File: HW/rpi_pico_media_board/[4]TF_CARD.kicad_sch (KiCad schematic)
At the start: 16 parts, among them J6 TF-01A

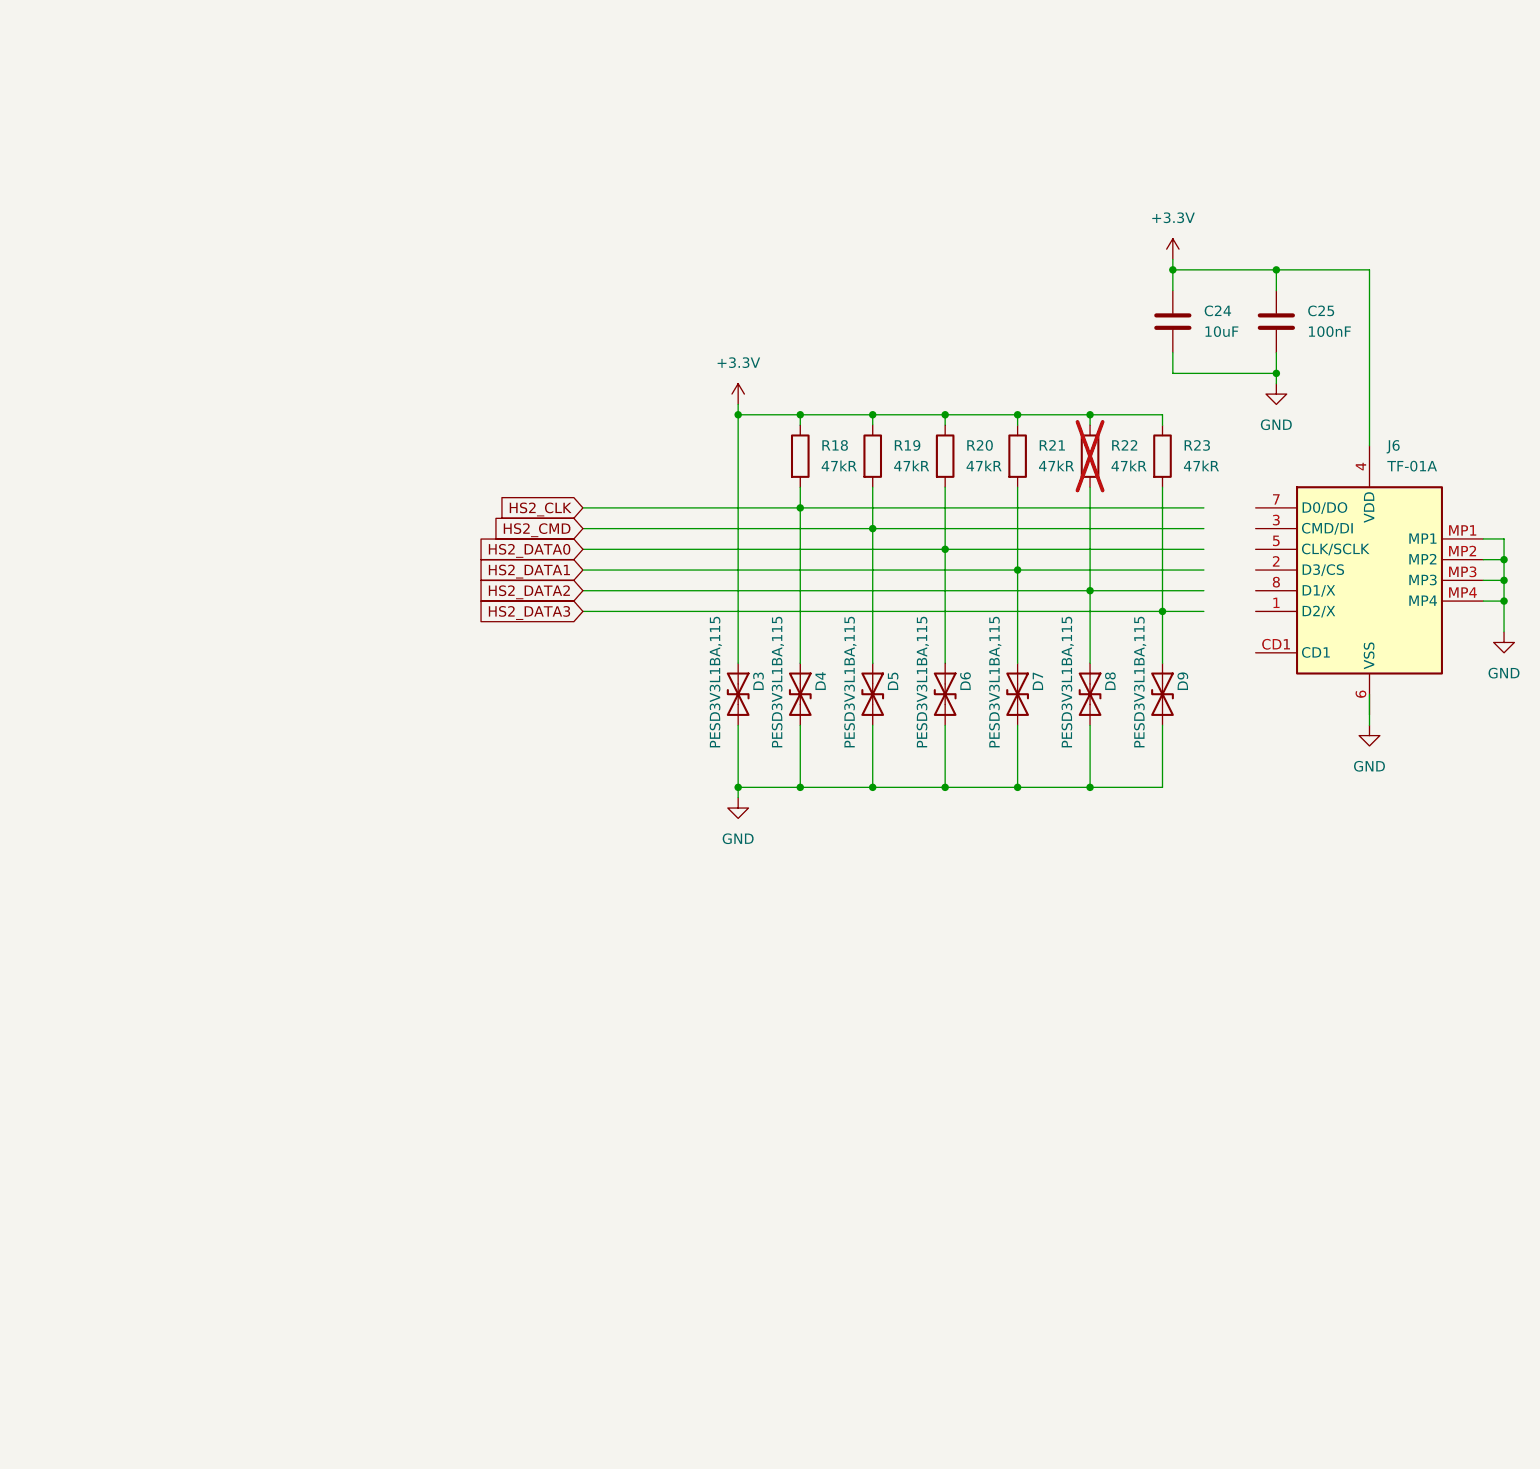
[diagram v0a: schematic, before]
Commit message: Scheme improvements
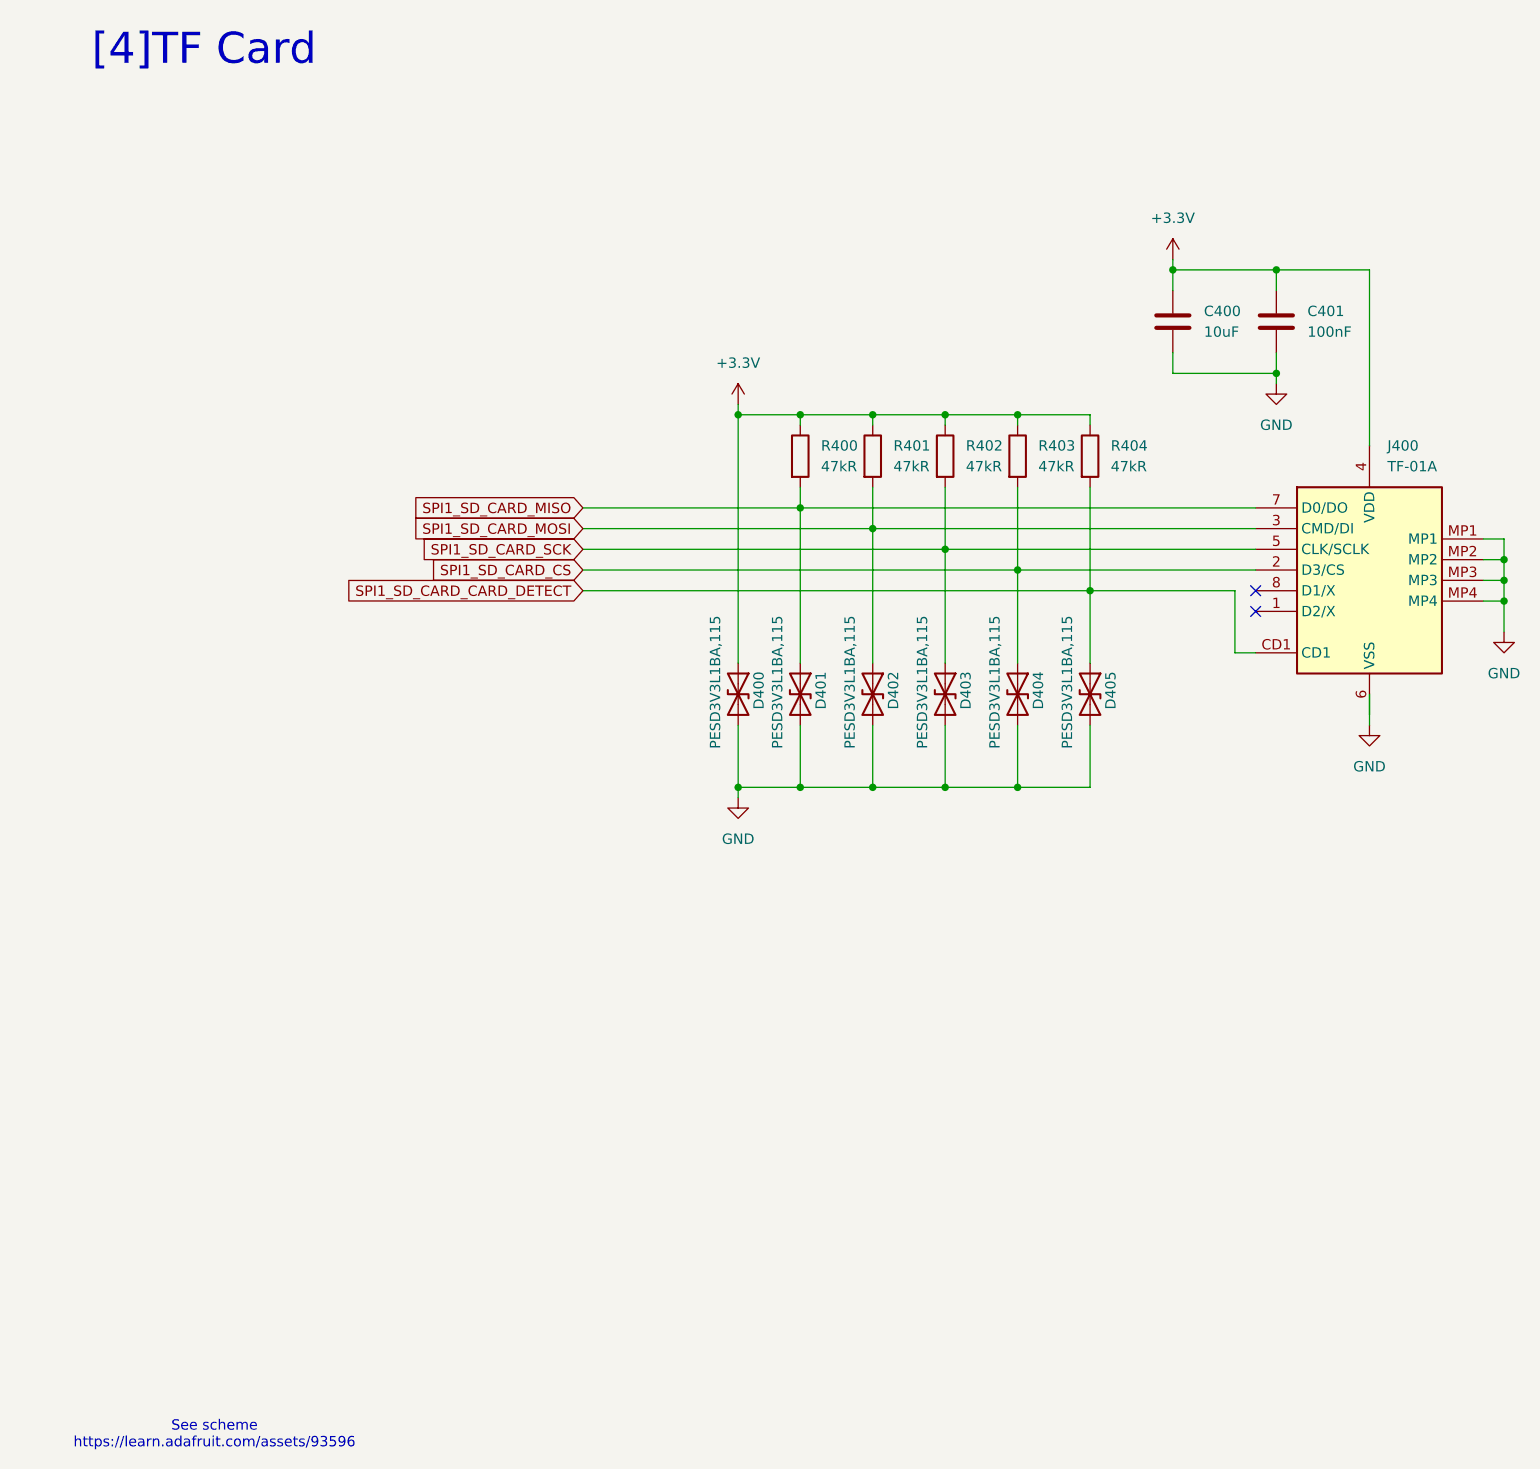
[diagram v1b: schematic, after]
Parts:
- removed D9: PESD3V3L1BA,115, Diode_SMD:D_SOD-323, symbol Device:D_TVS
- removed R23: 47kR, Resistor_SMD:R_0603_1608Metric, symbol Device:R
- R404: renamed from R22; now fitted
- renumbered C24 to C400, C25 to C401, D3 to D400, D4 to D401, D5 to D402, D6 to D403, D7 to D404, D8 to D405, J6 to J400, R18 to R400, R19 to R401, R20 to R402, R21 to R403
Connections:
- net HS2_CLK is gone; now on net SPI1_SD_CARD_MISO: D401.1 (A1), R400.2
- net HS2_CMD is gone; now on net SPI1_SD_CARD_MOSI: D402.1 (A1), R401.2
- net HS2_DATA0 is gone; now on net SPI1_SD_CARD_SCK: D403.1 (A1), R402.2
- net HS2_DATA1 is gone; now on net SPI1_SD_CARD_CS: D404.1 (A1), R403.2
- net HS2_DATA2 is gone; now on net SPI1_SD_CARD_CARD_DETECT: D405.1 (A1), R404.2
- net SPI1_SD_CARD_CS: now reaches J400.2 (D3/CS)
- net SPI1_SD_CARD_MOSI: now reaches J400.3 (CMD/DI)
- net SPI1_SD_CARD_SCK: now reaches J400.5 (CLK/SCLK)
- net SPI1_SD_CARD_MISO: now reaches J400.7 (D0/DO)
- net SPI1_SD_CARD_CARD_DETECT: now reaches J400.CD1
- no-connect marks 0 -> 2
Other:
- note added: "See scheme https://learn.adafruit.com/assets/93596"
- note added: "[4]TF Card"

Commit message: Minor BOM updates
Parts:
- J400: Manufacturer (none) -> Korean Hroparts Elec; Manufacturer Part Number (none) -> TF-01A; Manufacturer_Name Korean Hroparts Elec -> (none); Manufacturer_Part_Number TF-01A -> (none)
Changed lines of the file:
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@@
 			)
 		)
-		(property "Manufacturer_Name" "Korean Hroparts Elec"
+		(property "Manufacturer_Name" ""
 			(at 189.23 569.85 0)
 			(effects
@@
 			)
 		)
-		(property "Manufacturer_Part_Number" "TF-01A"
+		(property "Manufacturer_Part_Number" ""
 			(at 189.23 669.85 0)
 			(effects
@@
 				(hide yes)
 			)
+		)
+		(property "Manufacturer" "Korean Hroparts Elec"
+			(at 170.18 74.93 0)
+			(effects
+				(font
+					(size 1.27 1.27)
+				)
+				(hide yes)
+			)
+		)
+		(property "Manufacturer Part Number" "TF-01A"
+			(at 170.18 74.93 0)
+			(effects
+				(font
+					(size 1.27 1.27)
+				)
+				(hide yes)
+			)

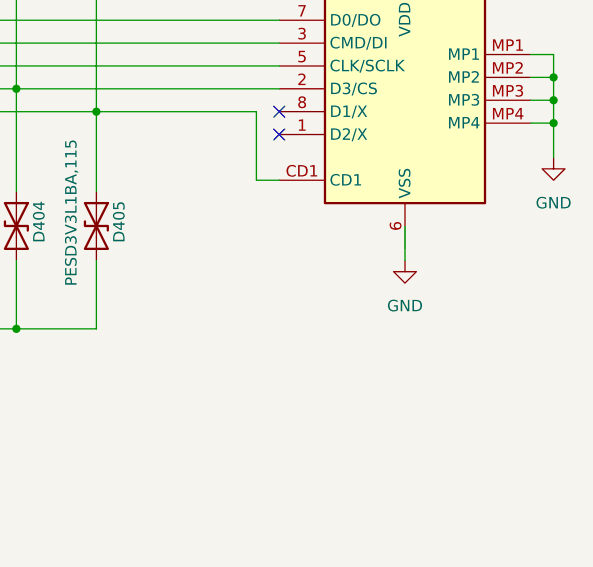
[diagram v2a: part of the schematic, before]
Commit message: DRC cleanup
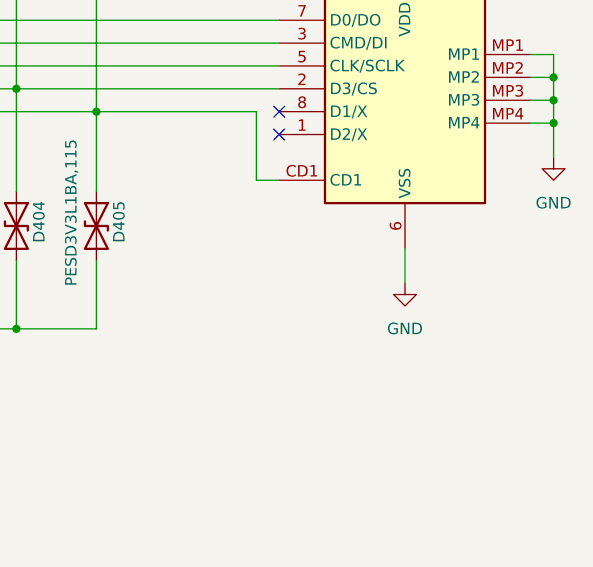
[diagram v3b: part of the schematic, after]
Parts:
- R404: Manufacturer Part Number 0805W8F4702T5E -> 0603WAJ0473T5E
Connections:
- net GND: now also J400.6 (VSS)
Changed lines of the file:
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@@
-	(wire
-		(pts
-			(xy 179.07 100.33) (xy 179.07 104.14)
-		)
-		(stroke
-			(width 0)
-			(type default)
-		)
-	)
 	(wire
 		(pts
@@
 		(pts
 			(xy 127 66.04) (xy 127 67.31)
+		)
+		(stroke
+			(width 0)
+			(type default)
+		)
+	)
+	(wire
+		(pts
+			(xy 179.07 102.87) (xy 179.07 106.68)
 		)
 		(stroke
@@
 		(lib_name "GND_3")
 		(lib_id "power:GND")
-		(at 179.07 104.14 0)
+		(at 179.07 106.68 0)
 		(unit 1)
 		(exclude_from_sim no)
@@
 		(fields_autoplaced yes)
 		(property "Reference" "#PWR38"
-			(at 179.07 110.49 0)
+			(at 179.07 113.03 0)
 			(effects
 				(font
@@
 		)
 		(property "Value" "GND"
-			(at 179.07 109.22 0)
+			(at 179.07 111.76 0)
 			(effects
 				(font
@@
 		)
 		(property "Footprint" ""
-			(at 179.07 104.14 0)
+			(at 179.07 106.68 0)
 			(effects
 				(font
@@
 		)
 		(property "Datasheet" ""
-			(at 179.07 104.14 0)
+			(at 179.07 106.68 0)
 			(effects
 				(font
@@
 		)
 		(property "Description" "Power symbol creates a global label with name \"GND\" , ground"
-			(at 179.07 104.14 0)
+			(at 179.07 106.68 0)
 			(effects
 				(font
@@
 			)
 		)
-		(property "Manufacturer Part Number" "0805W8F4702T5E"
+		(property "Manufacturer Part Number" "0603WAJ0473T5E"
 			(at 144.78 71.12 0)
 			(effects
